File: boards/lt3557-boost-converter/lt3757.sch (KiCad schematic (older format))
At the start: 22 parts, among them Q1 FDB86566, U1 LT3757

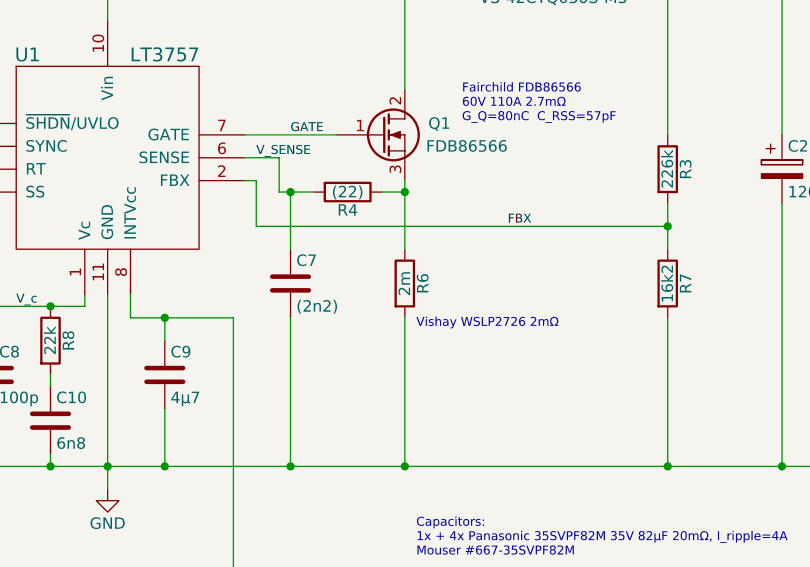
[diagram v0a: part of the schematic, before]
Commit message: lt3557-boost-converter: layout
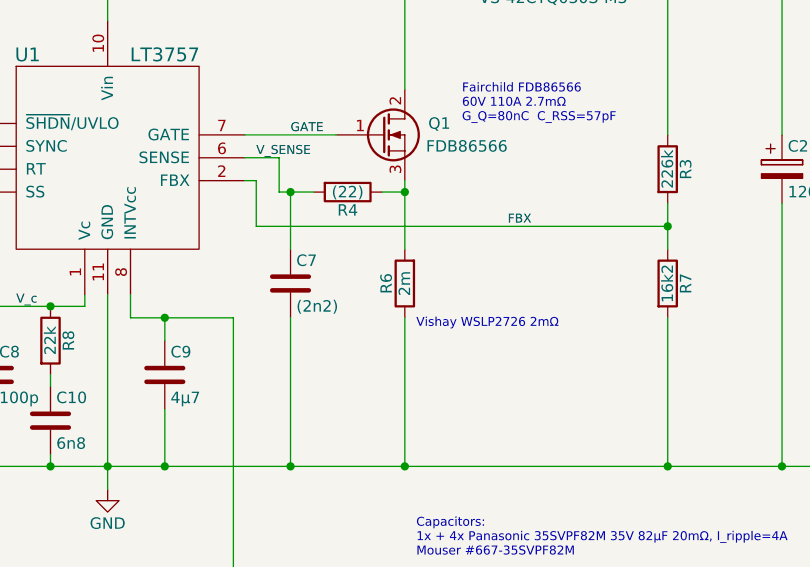
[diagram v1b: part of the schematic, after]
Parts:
- C5: footprint Capacitors_SMD:c_elec_10x10.5 -> Capacitors_SMD:c_elec_8x10.5
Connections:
- net GND: now also R6.1; no longer R6.2
- net at Q1.3 (S), R4.1: now also R6.2; no longer R6.1
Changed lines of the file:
@@
 F 3 "" H 5900 2650 50  0000 C CNN
 	1    5900 2650
-	1    0    0    -1
+	-1   0    0    1
 $EndComp
 $Comp
@@
 F 0 "C5" H 8625 2250 50  0000 L CNN
 F 1 "120µ" H 8625 2050 50  0000 L CNN
-F 2 "Capacitors_SMD:c_elec_10x10.5" H 8638 2000 50  0001 C CNN
+F 2 "Capacitors_SMD:c_elec_8x10.5" H 8638 2000 50  0001 C CNN
 F 3 "" H 8600 2150 50  0000 C CNN
 	1    8600 2150
